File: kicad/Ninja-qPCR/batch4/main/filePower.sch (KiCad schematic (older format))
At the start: 55 parts, among them J8 Barrel_Jack_Switch, J9 ATX-24, U1 DIN4_PWR, U2 IFX1763, U3 BD9D320EFJ-E2, U4 LTC3260EMSE-TRPBF, U5 CJT1117-3.3

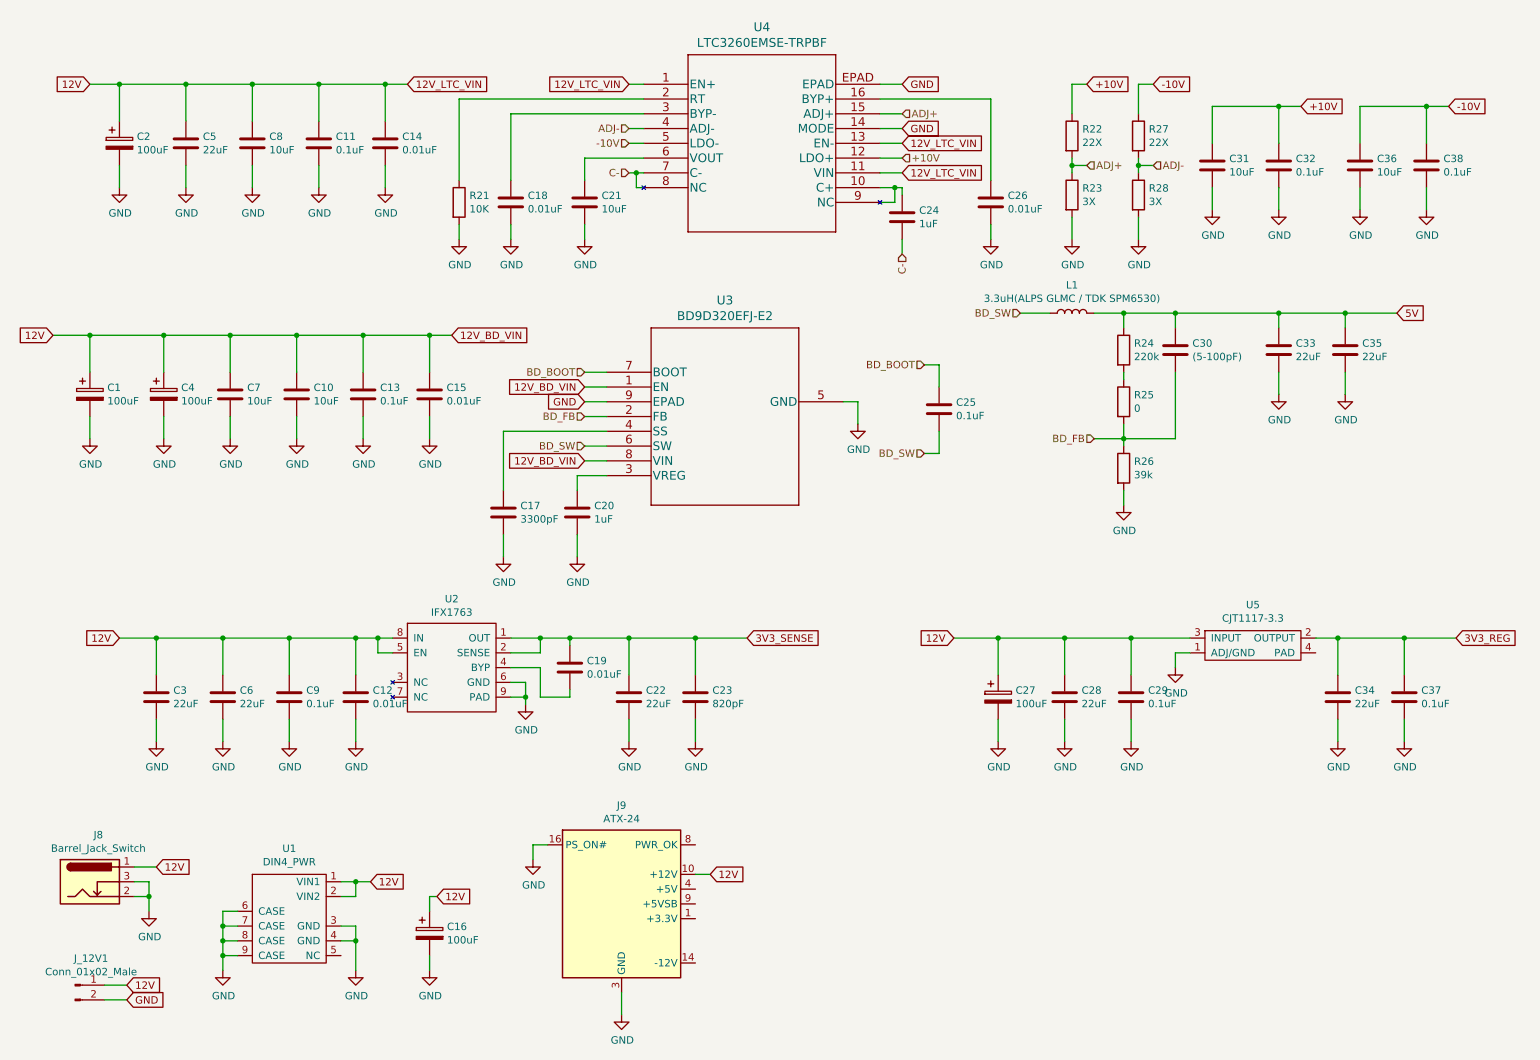
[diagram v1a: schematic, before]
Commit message: buildup batch4/main
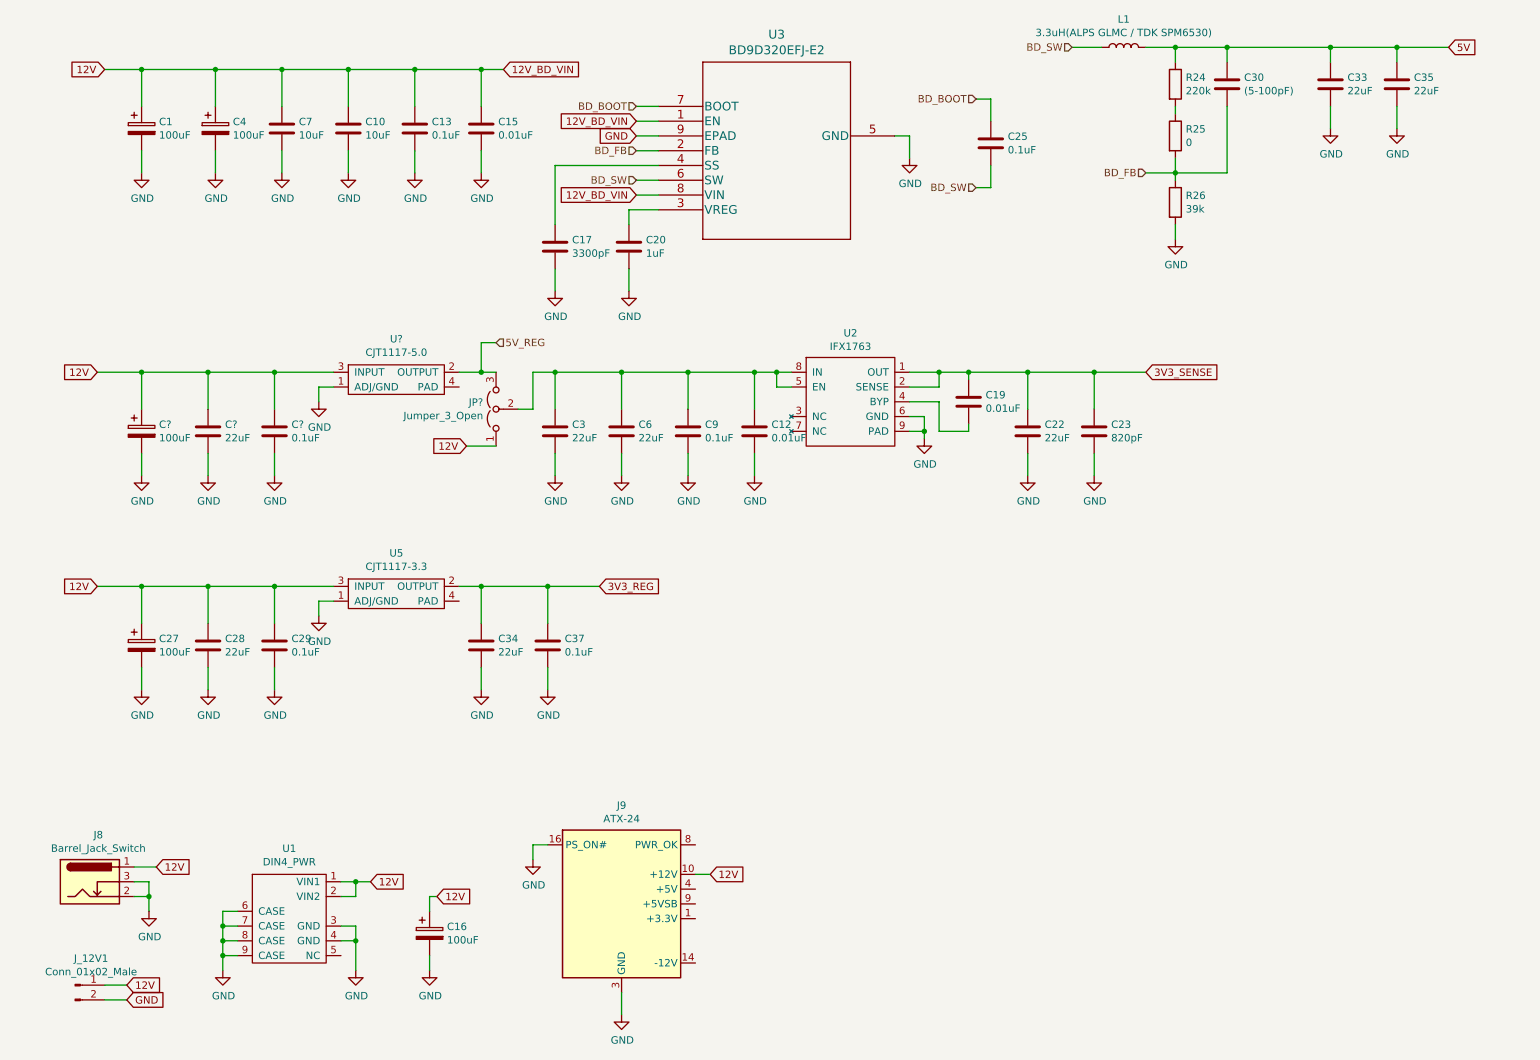
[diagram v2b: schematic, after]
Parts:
- removed C11, C32, C38: 0.1uF, Capacitors_SMD:C_0805_HandSoldering, symbol Device:C
- removed C14, C18, C26: 0.01uF, Capacitors_SMD:C_0603_HandSoldering, symbol Device:C
- removed C2: 100uF, Capacitors_SMD:CP_Elec_6.3x5.8, symbol Device:CP
- removed C21, C31, C36, C8: 10uF, Capacitors_SMD:C_0805_HandSoldering, symbol Device:C
- removed C24: 1uF, Capacitors_SMD:C_0805_HandSoldering, symbol Device:C
- removed C5: 22uF, Capacitors_SMD:C_0805_HandSoldering, symbol Device:C
- removed R21: 10K, Resistors_SMD:R_0603_HandSoldering, symbol Device:R
- removed R22, R27: 22X, Resistors_SMD:R_0603_HandSoldering, symbol Device:R
- removed R23, R28: 3X, Resistors_SMD:R_0603_HandSoldering, symbol Device:R
- removed U4: LTC3260EMSE-TRPBF, Ninja-qPCR:LTC3260EMSE-TRPBF, symbol Ninja-qPCR:LTC3260EMSE-TRPBF
- added C?: 22uF, Capacitors_SMD:C_0805_HandSoldering, symbol Device:C
- added C?: 0.1uF, Capacitors_SMD:C_0805_HandSoldering, symbol Device:C
- added C?: 100uF, Capacitors_SMD:CP_Elec_6.3x5.8, symbol Device:CP
- added JP?: Jumper_3_Open, symbol Jumper:Jumper_3_Open
- added U?: CJT1117-5.0, symbol Ninja-qPCR:CJT1117-5.0
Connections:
- net 12V: now also C?.1, C?.1, C?.1, JP?.1 (A), U?.3 (INPUT); no longer C12.1, C3.1, C6.1, C9.1, U2.5 (EN), U2.8 (IN)
- net GND: now also C?.2, C?.2, C?.2, U?.1 (ADJ/GND)
- new net: C12.1, C3.1, C6.1, C9.1, JP?.2 (C), U2.5 (EN), U2.8 (IN)
- new net 5V_REG: JP?.3 (B), U?.2 (OUTPUT)
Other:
- moved on the sheet: C1, C10, C12, C13, C15, C17, C19, C20, C22, C23, C25, C27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
